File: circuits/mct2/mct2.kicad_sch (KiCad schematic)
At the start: 16 parts

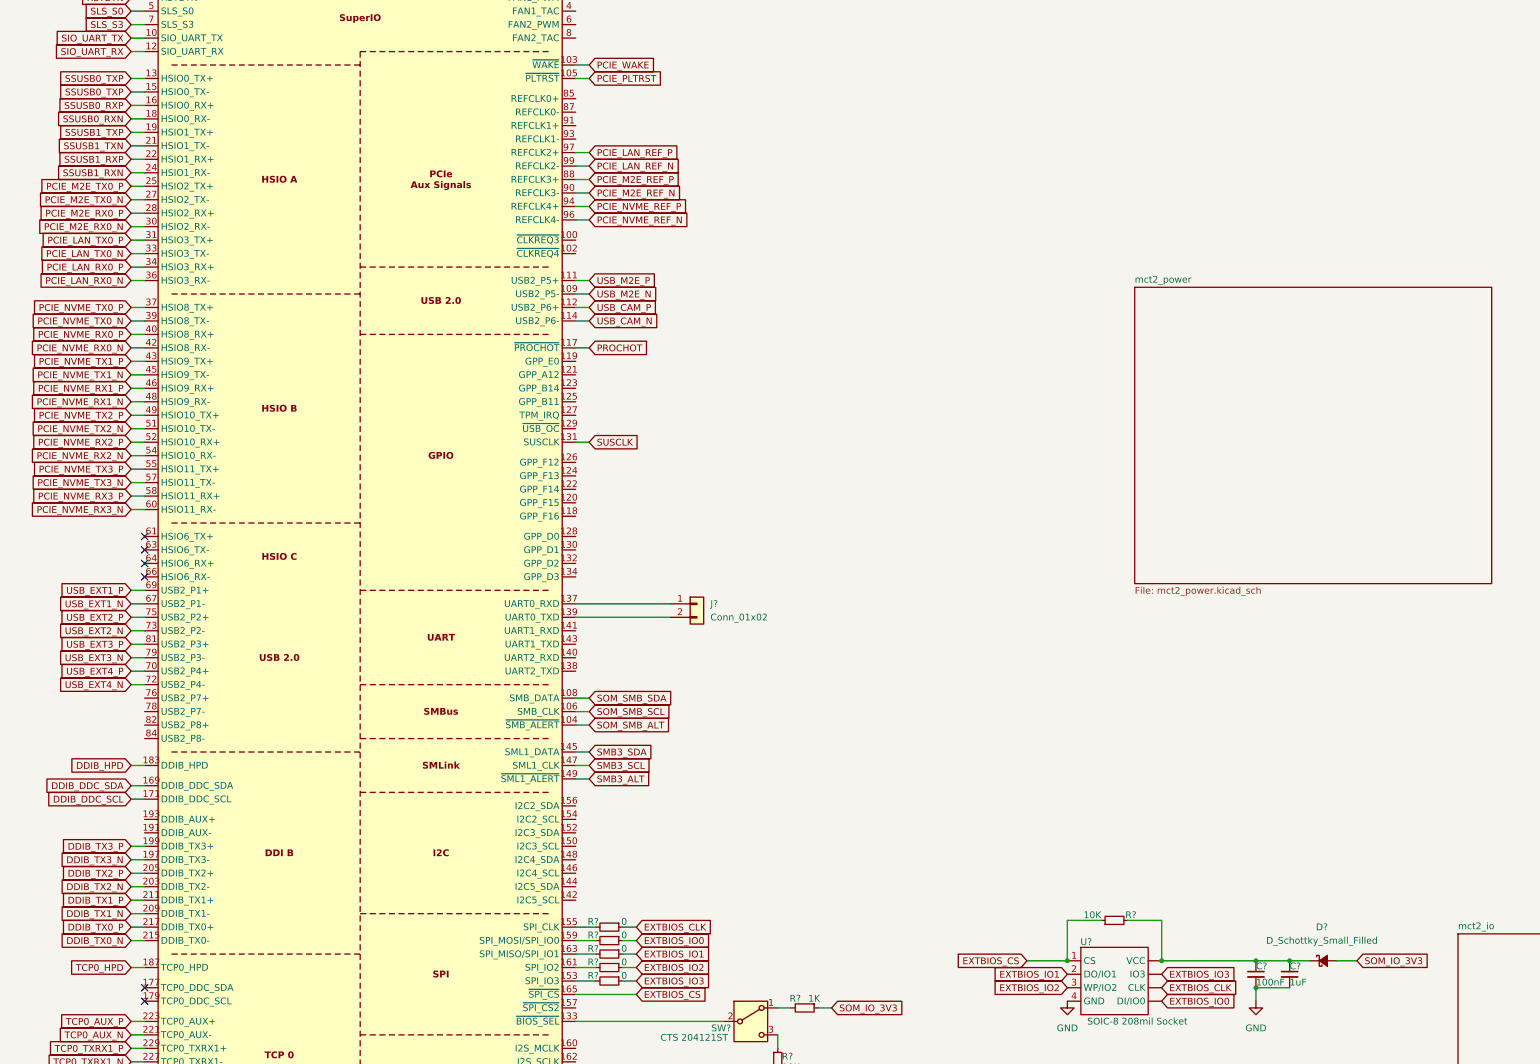
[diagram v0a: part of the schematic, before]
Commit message: Aug 17, 2024
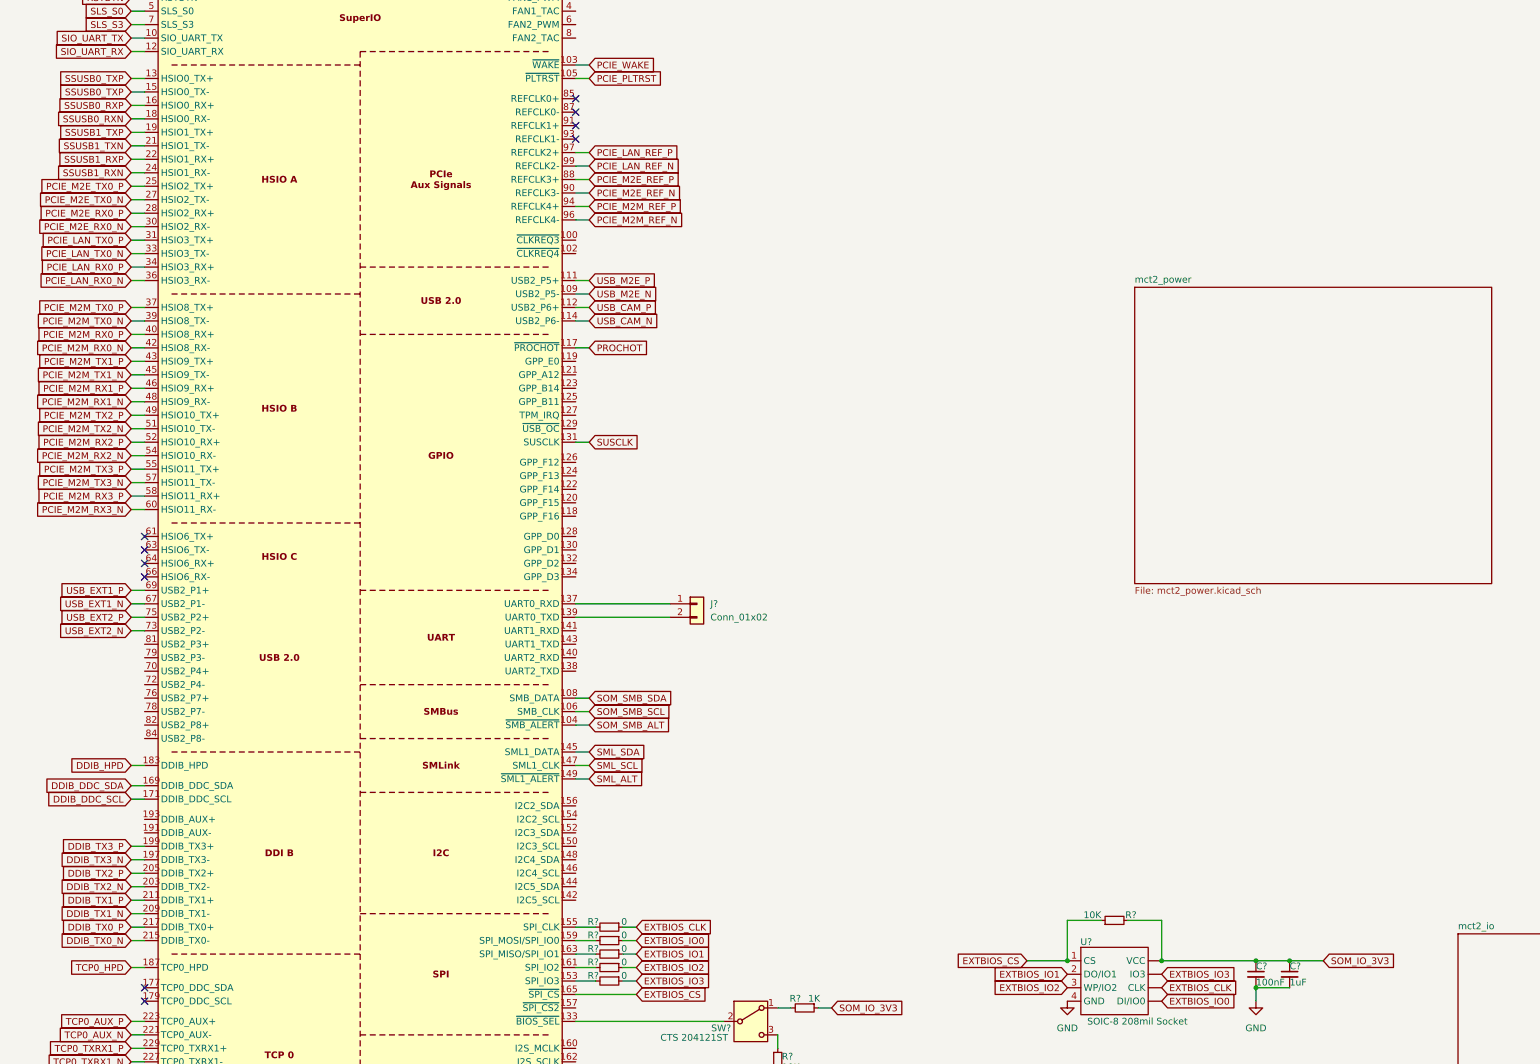
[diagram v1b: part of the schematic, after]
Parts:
- removed D?: D_Schottky_Small_Filled, symbol Device:D_Schottky_Small_Filled
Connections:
- net SOM_IO_3V3: now also C?.1, C?.1, R?.2, U?. (VCC)
- net PCIE_NVME_REF_N renamed PCIE_M2M_REF_N
- net PCIE_NVME_REF_P renamed PCIE_M2M_REF_P
- net PCIE_NVME_RX0_N renamed PCIE_M2M_RX0_N
- net PCIE_NVME_RX0_P renamed PCIE_M2M_RX0_P
- net PCIE_NVME_RX1_N renamed PCIE_M2M_RX1_N
- net PCIE_NVME_RX1_P renamed PCIE_M2M_RX1_P
- net PCIE_NVME_RX2_N renamed PCIE_M2M_RX2_N
- net PCIE_NVME_RX2_P renamed PCIE_M2M_RX2_P
- net PCIE_NVME_RX3_N renamed PCIE_M2M_RX3_N
- net PCIE_NVME_RX3_P renamed PCIE_M2M_RX3_P
- net PCIE_NVME_TX0_N renamed PCIE_M2M_TX0_N
- net PCIE_NVME_TX0_P renamed PCIE_M2M_TX0_P
- net PCIE_NVME_TX1_N renamed PCIE_M2M_TX1_N
- net PCIE_NVME_TX1_P renamed PCIE_M2M_TX1_P
- net PCIE_NVME_TX2_N renamed PCIE_M2M_TX2_N
- net PCIE_NVME_TX2_P renamed PCIE_M2M_TX2_P
- net PCIE_NVME_TX3_N renamed PCIE_M2M_TX3_N
- net PCIE_NVME_TX3_P renamed PCIE_M2M_TX3_P
- net SMB3_ALT renamed SML_ALT
- net SMB3_SCL renamed SML_SCL
- net SMB3_SDA renamed SML_SDA
- net USB_EXT3_N: no longer names the net of A1.79 (USB2_P3-)
- net USB_EXT3_P: no longer names the net of A1.81 (USB2_P3+)
- net USB_EXT4_N: no longer names the net of A1.72 (USB2_P4-)
- net USB_EXT4_P: no longer names the net of A1.70 (USB2_P4+)
- no-connect marks 8 -> 12

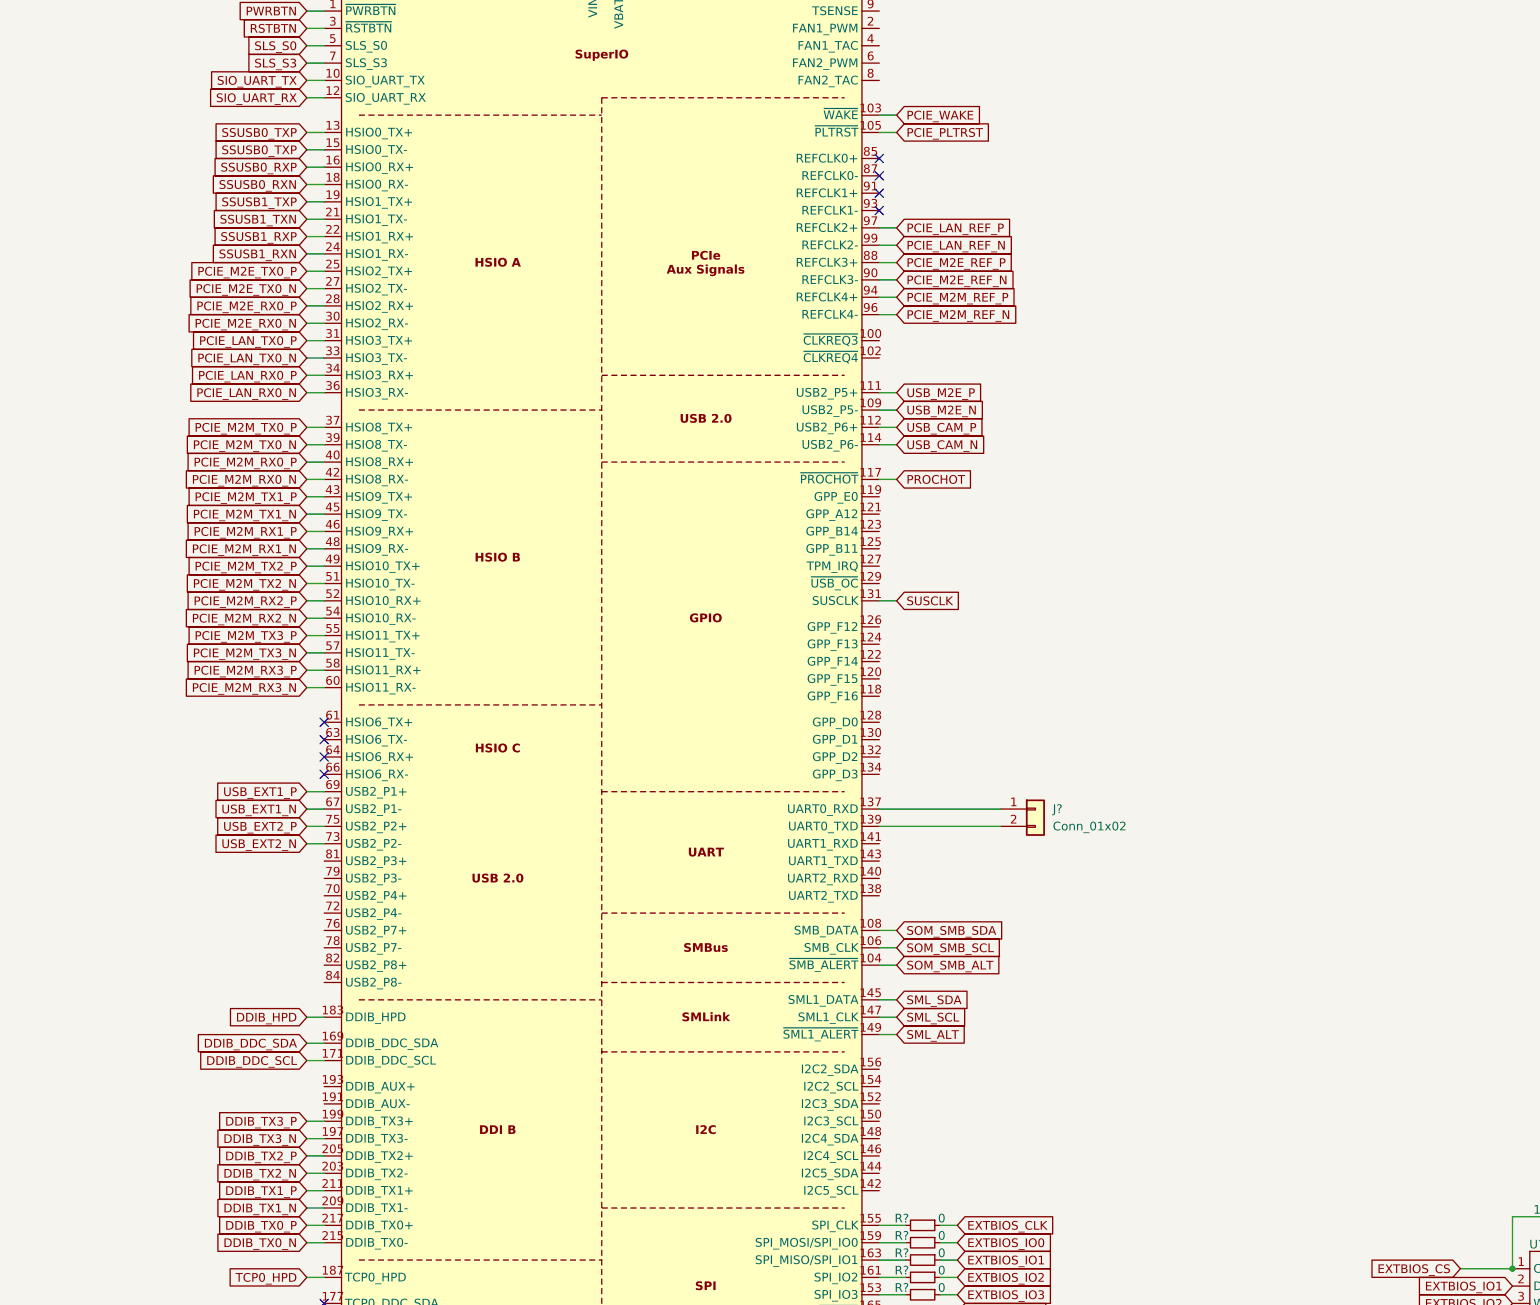
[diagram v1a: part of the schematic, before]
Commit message: Aug 17, 2024 2
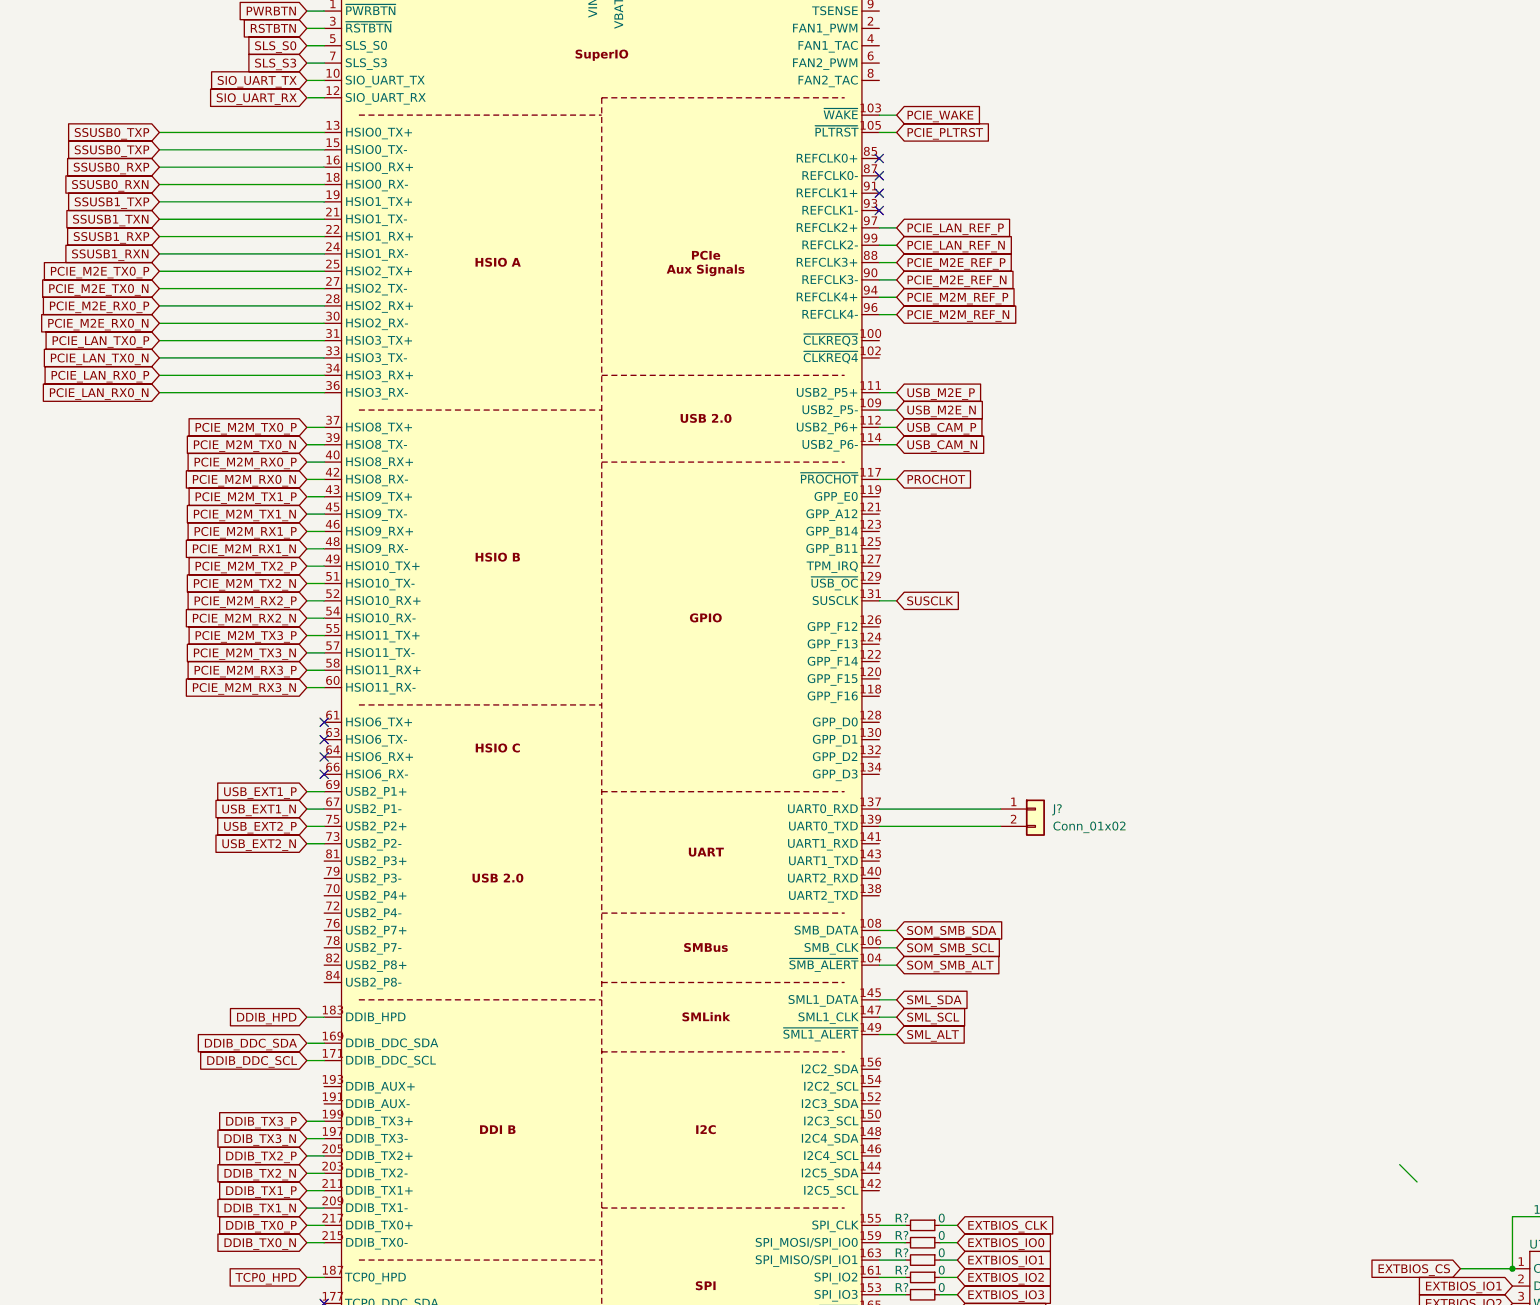
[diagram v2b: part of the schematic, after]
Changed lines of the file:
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@@
 		(at 501.65 537.21)
 	)
+	(bus_entry
+		(at 659.13 516.89)
+		(size 2.54 2.54)
+		(stroke
+			(width 0)
+			(type default)
+		)
+	)
 	(wire
 		(pts
@@
 	(wire
 		(pts
-			(xy 499.11 381) (xy 501.65 381)
+			(xy 477.52 381) (xy 501.65 381)
 		)
 		(stroke
@@
 	(wire
 		(pts
-			(xy 499.11 388.62) (xy 501.65 388.62)
+			(xy 477.52 388.62) (xy 501.65 388.62)
 		)
 		(stroke
@@
 	(wire
 		(pts
-			(xy 499.11 393.7) (xy 501.65 393.7)
+			(xy 477.52 393.7) (xy 501.65 393.7)
 		)
 		(stroke
@@
 	(wire
 		(pts
-			(xy 499.11 403.86) (xy 501.65 403.86)
+			(xy 477.52 403.86) (xy 501.65 403.86)
 		)
 		(stroke
@@
 	(wire
 		(pts
-			(xy 499.11 365.76) (xy 501.65 365.76)
+			(xy 477.52 365.76) (xy 501.65 365.76)
 		)
 		(stroke
@@
 	(wire
 		(pts
-			(xy 499.11 398.78) (xy 501.65 398.78)
+			(xy 477.52 398.78) (xy 501.65 398.78)
 		)
 		(stroke
@@
 	(wire
 		(pts
-			(xy 499.11 401.32) (xy 501.65 401.32)
+			(xy 477.52 401.32) (xy 501.65 401.32)
 		)
 		(stroke
@@
 	(wire
 		(pts
-			(xy 499.11 368.3) (xy 501.65 368.3)
+			(xy 477.52 368.3) (xy 501.65 368.3)
 		)
 		(stroke
@@
 	(wire
 		(pts
-			(xy 499.11 375.92) (xy 501.65 375.92)
+			(xy 477.52 375.92) (xy 501.65 375.92)
 		)
 		(stroke
@@
 	(wire
 		(pts
-			(xy 499.11 370.84) (xy 501.65 370.84)
+			(xy 477.52 370.84) (xy 501.65 370.84)
 		)
 		(stroke
@@
 	(wire
 		(pts
-			(xy 499.11 386.08) (xy 501.65 386.08)
+			(xy 477.52 386.08) (xy 501.65 386.08)
 		)
 		(stroke
@@
 	(wire
 		(pts
-			(xy 499.11 391.16) (xy 501.65 391.16)
+			(xy 477.52 391.16) (xy 501.65 391.16)
 		)
 		(stroke
@@
 	(wire
 		(pts
-			(xy 499.11 373.38) (xy 501.65 373.38)
+			(xy 477.52 373.38) (xy 501.65 373.38)
 		)
 		(stroke
@@
 	(wire
 		(pts
-			(xy 499.11 378.46) (xy 501.65 378.46)
+			(xy 477.52 378.46) (xy 501.65 378.46)
 		)
 		(stroke
@@
 	(wire
 		(pts
-			(xy 499.11 383.54) (xy 501.65 383.54)
+			(xy 477.52 383.54) (xy 501.65 383.54)
 		)
 		(stroke
@@
 	(wire
 		(pts
-			(xy 499.11 396.24) (xy 501.65 396.24)
+			(xy 477.52 396.24) (xy 501.65 396.24)
 		)
 		(stroke
@@
 	(global_label "SSUSB1_RXN"
 		(shape input)
-		(at 499.11 383.54 180)
+		(at 477.52 383.54 180)
 		(fields_autoplaced yes)
 		(effects
@@
 		)
 		(property "Intersheetrefs" "${INTERSHEET_REFS}"
-			(at 483.9087 383.54 0)
+			(at 462.3187 383.54 0)
 			(effects
 				(font
@@
 	(global_label "PCIE_M2E_TX0_P"
 		(shape input)
-		(at 499.11 386.08 180)
+		(at 477.52 386.08 180)
 		(fields_autoplaced yes)
 		(effects
@@
 		)
 		(property "Intersheetrefs" "${INTERSHEET_REFS}"
-			(at 483.1226 386.08 0)
+			(at 461.5326 386.08 0)
 			(effects
 				(font
@@
 	(global_label "PCIE_M2E_RX0_P"
 		(shape input)
-		(at 499.11 391.16 180)
+		(at 477.52 391.16 180)
 		(fields_autoplaced yes)
 		(effects
@@
 		)
 		(property "Intersheetrefs" "${INTERSHEET_REFS}"
-			(at 482.8202 391.16 0)
+			(at 461.2302 391.16 0)
 			(effects
 				(font
@@
 	(global_label "PCIE_M2E_TX0_N"
 		(shape input)
-		(at 499.11 388.62 180)
+		(at 477.52 388.62 180)
 		(fields_autoplaced yes)
 		(effects
@@
 		)
 		(property "Intersheetrefs" "${INTERSHEET_REFS}"
-			(at 483.0621 388.62 0)
+			(at 461.4721 388.62 0)
 			(effects
 				(font
@@
 	(global_label "SSUSB1_TXP"
 		(shape input)
-		(at 499.11 375.92 180)
+		(at 477.52 375.92 180)
 		(fields_autoplaced yes)
 		(effects
@@
 		)
 		(property "Intersheetrefs" "${INTERSHEET_REFS}"
-			(at 484.2716 375.92 0)
+			(at 462.6816 375.92 0)
 			(effects
 				(font
@@
 	(global_label "SSUSB1_RXP"
 		(shape input)
-		(at 499.11 381 180)
+		(at 477.52 381 180)
 		(fields_autoplaced yes)
 		(effects
@@
 		)
 		(property "Intersheetrefs" "${INTERSHEET_REFS}"
-			(at 484.2716 381 0)
+			(at 462.6816 381 0)
 			(effects
 				(font
@@
 	(global_label "PCIE_LAN_RX0_P"
 		(shape input)
-		(at 499.11 401.32 180)
+		(at 477.52 401.32 180)
 		(fields_autoplaced yes)
 		(effects
@@
 		)
 		(property "Intersheetrefs" "${INTERSHEET_REFS}"
-			(at 482.8202 401.32 0)
+			(at 461.2302 401.32 0)
 			(effects
 				(font
@@
 	(global_label "SSUSB0_TXP"
 		(shape input)
-		(at 499.11 368.3 180)
+		(at 477.52 368.3 180)
 		(fields_autoplaced yes)
 		(effects
@@
 		)
 		(property "Intersheetrefs" "${INTERSHEET_REFS}"
-			(at 484.2716 368.3 0)
+			(at 462.6816 368.3 0)
 			(effects
 				(font
@@
 	(global_label "SSUSB0_RXN"
 		(shape input)
-		(at 499.11 373.38 180)
+		(at 477.52 373.38 180)
 		(fields_autoplaced yes)
 		(effects
@@
 		)
 		(property "Intersheetrefs" "${INTERSHEET_REFS}"
-			(at 483.9087 373.38 0)
+			(at 462.3187 373.38 0)
 			(effects
 				(font
@@
 	(global_label "PCIE_LAN_TX0_P"
 		(shape input)
-		(at 499.11 396.24 180)
+		(at 477.52 396.24 180)
 		(fields_autoplaced yes)
 		(effects
@@
 		)
 		(property "Intersheetrefs" "${INTERSHEET_REFS}"
-			(at 483.1226 396.24 0)
+			(at 461.5326 396.24 0)
 			(effects
 				(font
@@
 	(global_label "SSUSB0_TXP"
 		(shape input)
-		(at 499.11 365.76 180)
+		(at 477.52 365.76 180)
 		(fields_autoplaced yes)
 		(effects
@@
 		)
 		(property "Intersheetrefs" "${INTERSHEET_REFS}"
-			(at 484.2716 365.76 0)
+			(at 462.6816 365.76 0)
 			(effects
 				(font
@@
 	(global_label "PCIE_M2E_RX0_N"
 		(shape input)
-		(at 499.11 393.7 180)
+		(at 477.52 393.7 180)
 		(fields_autoplaced yes)
 		(effects
@@
 		)
 		(property "Intersheetrefs" "${INTERSHEET_REFS}"
-			(at 482.7597 393.7 0)
+			(at 461.1697 393.7 0)
 			(effects
 				(font
@@
 	(global_label "PCIE_LAN_RX0_N"
 		(shape input)
-		(at 499.11 403.86 180)
+		(at 477.52 403.86 180)
 		(fields_autoplaced yes)
 		(effects
@@
 		)
 		(property "Intersheetrefs" "${INTERSHEET_REFS}"
-			(at 482.7597 403.86 0)
+			(at 461.1697 403.86 0)
 			(effects
 				(font
@@
 	(global_label "SSUSB0_RXP"
 		(shape input)
-		(at 499.11 370.84 180)
+		(at 477.52 370.84 180)
 		(fields_autoplaced yes)
 		(effects
@@
 		)
 		(property "Intersheetrefs" "${INTERSHEET_REFS}"
-			(at 484.2716 370.84 0)
+			(at 462.6816 370.84 0)
 			(effects
 				(font
@@
 	(global_label "SSUSB1_TXN"
 		(shape input)
-		(at 499.11 378.46 180)
+		(at 477.52 378.46 180)
 		(fields_autoplaced yes)
 		(effects
@@
 		)
 		(property "Intersheetrefs" "${INTERSHEET_REFS}"
-			(at 484.2111 378.46 0)
+			(at 462.6211 378.46 0)
 			(effects
 				(font
@@
 	(global_label "PCIE_LAN_TX0_N"
 		(shape input)
-		(at 499.11 398.78 180)
+		(at 477.52 398.78 180)
 		(fields_autoplaced yes)
 		(effects
@@
 		)
 		(property "Intersheetrefs" "${INTERSHEET_REFS}"
-			(at 483.0621 398.78 0)
+			(at 461.4721 398.78 0)
 			(effects
 				(font
